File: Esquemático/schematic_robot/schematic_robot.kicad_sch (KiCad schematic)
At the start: 19 parts, among them J1 Conn_01x04_Pin, J2 Conn_01x01_Socket, J3 Conn_01x01_Socket, J4 Conn_01x01_Socket, J5 Conn_01x01_Socket, J6 Conn_01x01_Socket, J7 Conn_01x01_Socket, J8 Conn_01x01_Socket, J9 Conn_01x01_Socket, M1 Motor_Servo, M2 Motor_Servo, M3 Motor_Servo, M4 Motor_Servo, M5 Motor_Servo, U1 TB6600, U2 ESP32-WROOM-32, U3 PCA9685PW

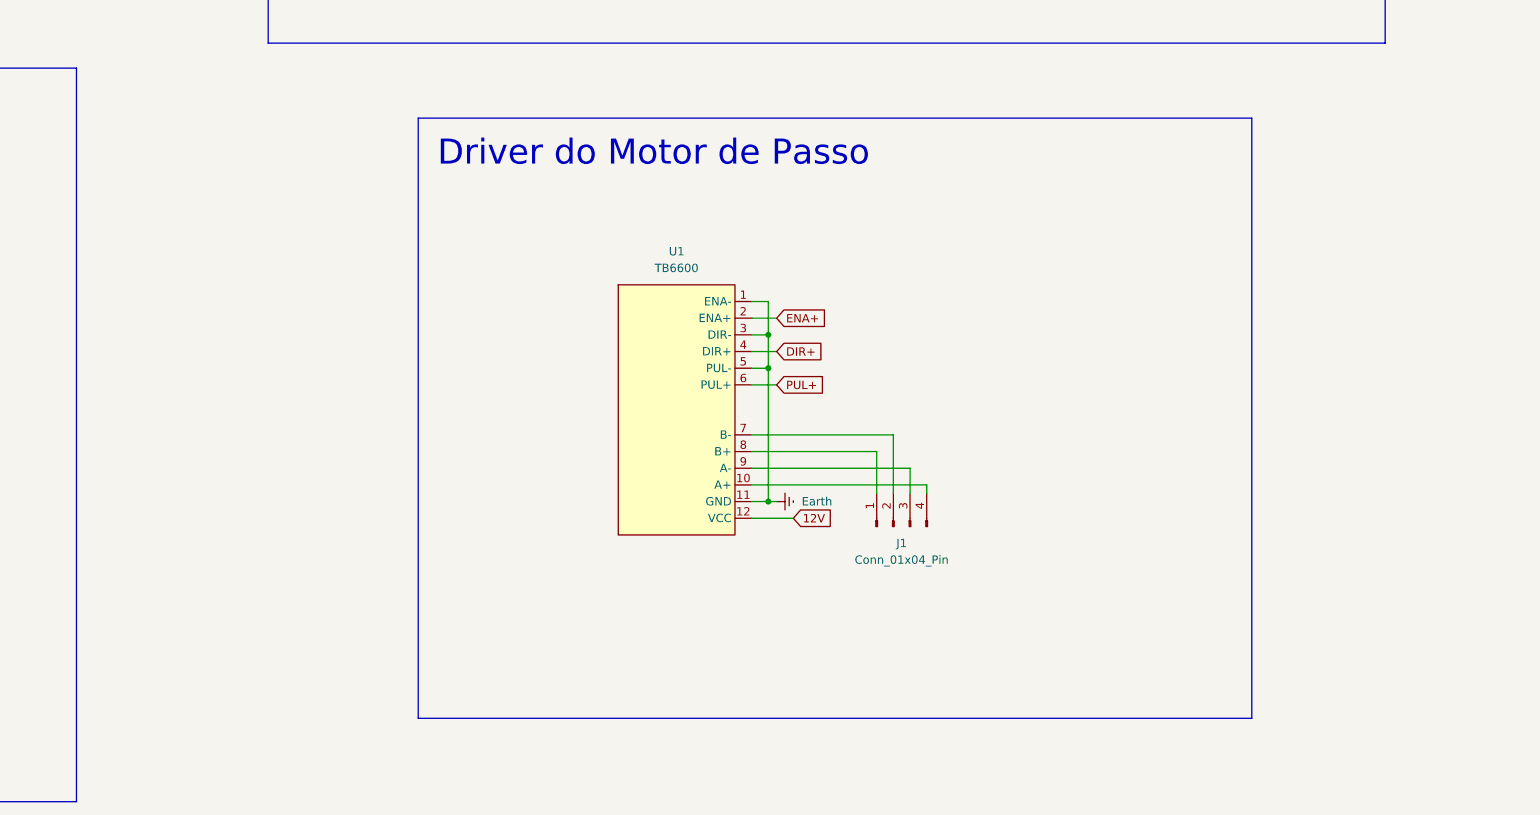
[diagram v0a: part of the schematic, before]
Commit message: Upload da luva
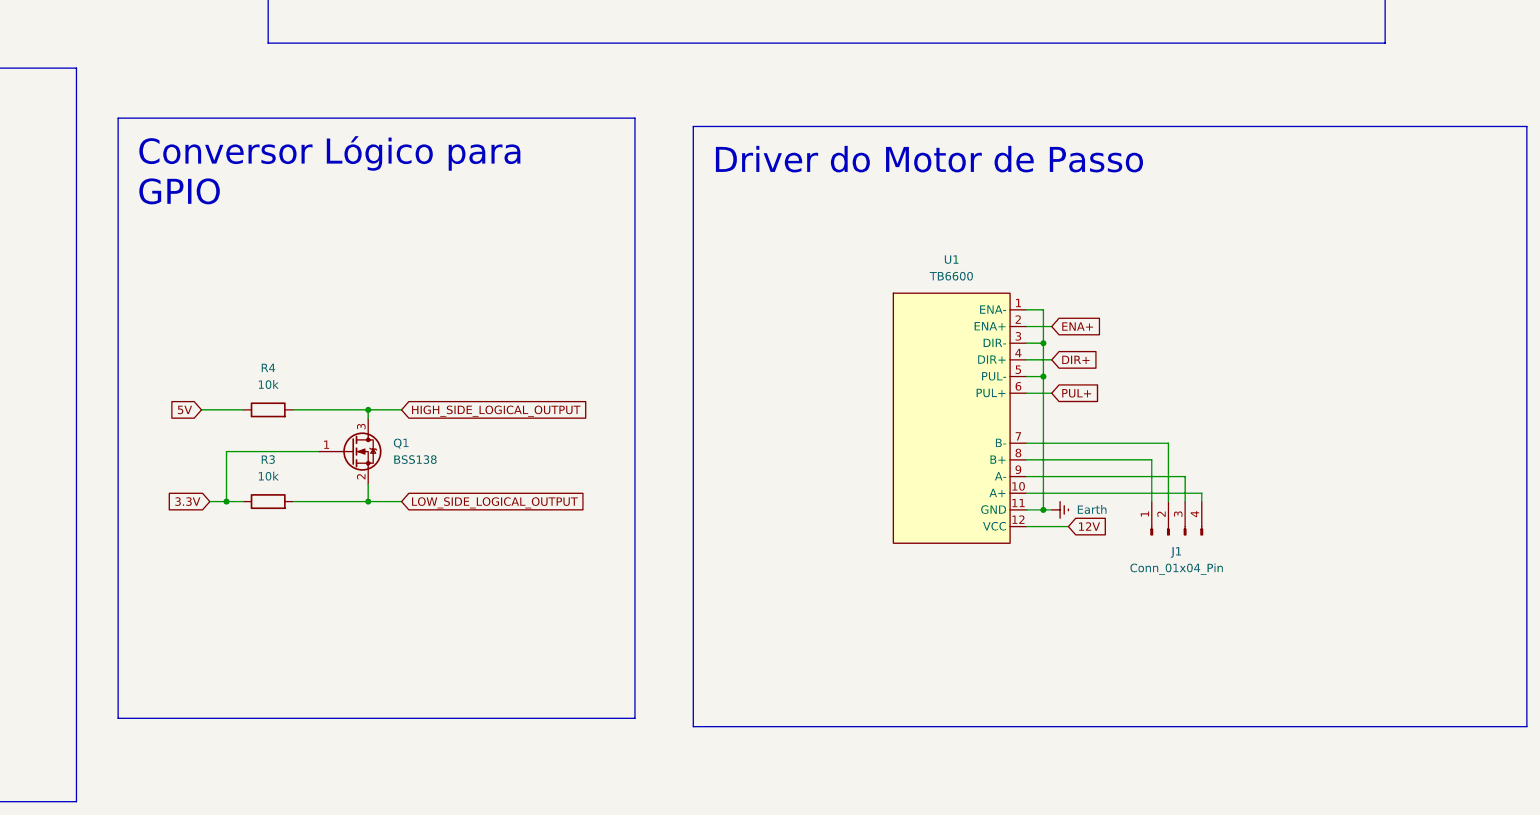
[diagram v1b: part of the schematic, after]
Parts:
- added Q1: BSS138, Package_TO_SOT_SMD:SOT-23, symbol Transistor_FET:BSS138
- added R3, R4: 10k, symbol Device:R
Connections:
- net 5V: now also R4.1
- new net 3.3V: Q1.1 (G), R3.1
- new net HIGH_SIDE_LOGICAL_OUTPUT: Q1.3 (D), R4.2
- new net LOW_SIDE_LOGICAL_OUTPUT: Q1.2 (S), R3.2
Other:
- moved on the sheet: J1, U1
